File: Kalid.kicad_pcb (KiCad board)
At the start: 4 copper layers, 90 x 40 mm, 160 parts, among them J1 USB_A, J2 USB_C_Receptacle_USB2.0_16P, J3 USB_A, J31 DC Connector, J4 USB_A, J5 USB_A, J6 Conn_01x04, J7 USB_C_Receptacle_USB2.0_16P, U1 TPS62933, U2 TPS62933, U3 GL3523-OTY30, U4 USB-PD, U5 LPW5209AB5F, U6 LPW5209AB5F, U7 LPW5209AB5F, U8 LPW5209AB5F, U9 MX25L1006EMI-10G, Y1 Crystal 25MHz 2016

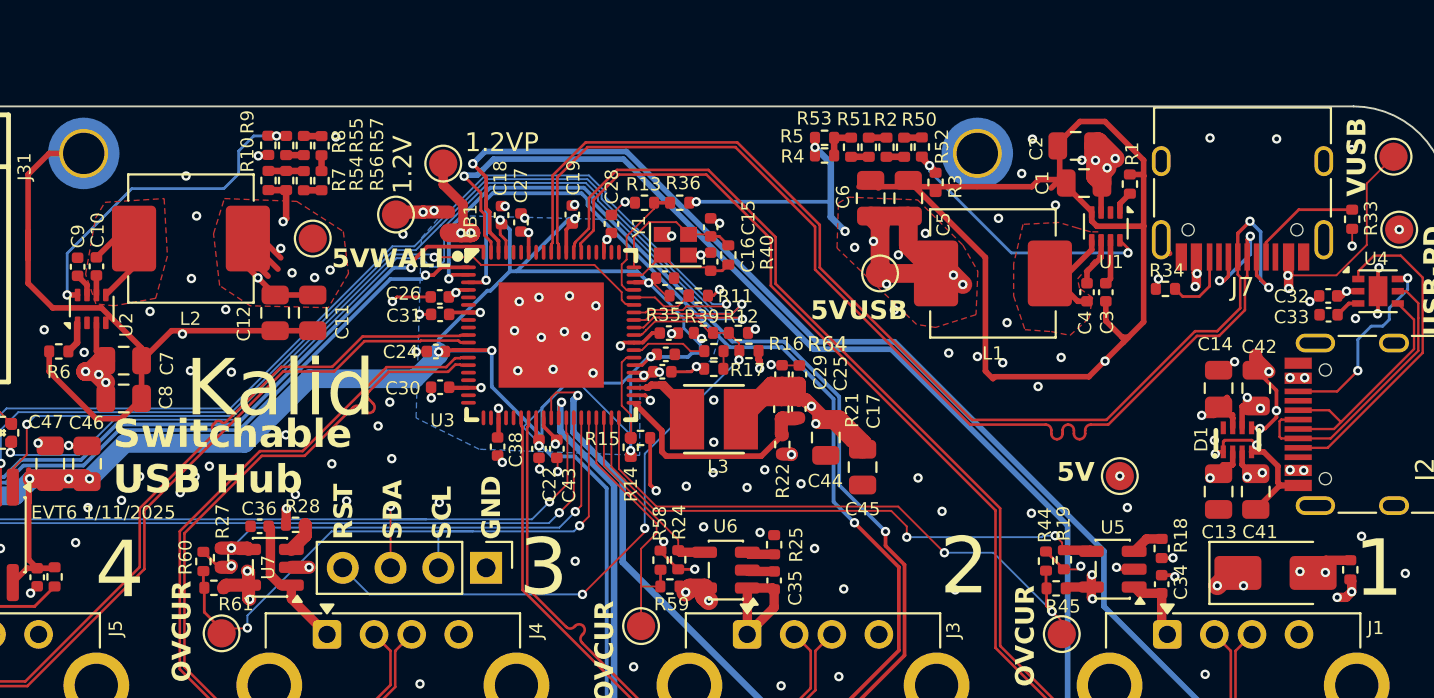
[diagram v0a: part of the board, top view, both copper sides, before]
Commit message: evt5: Release
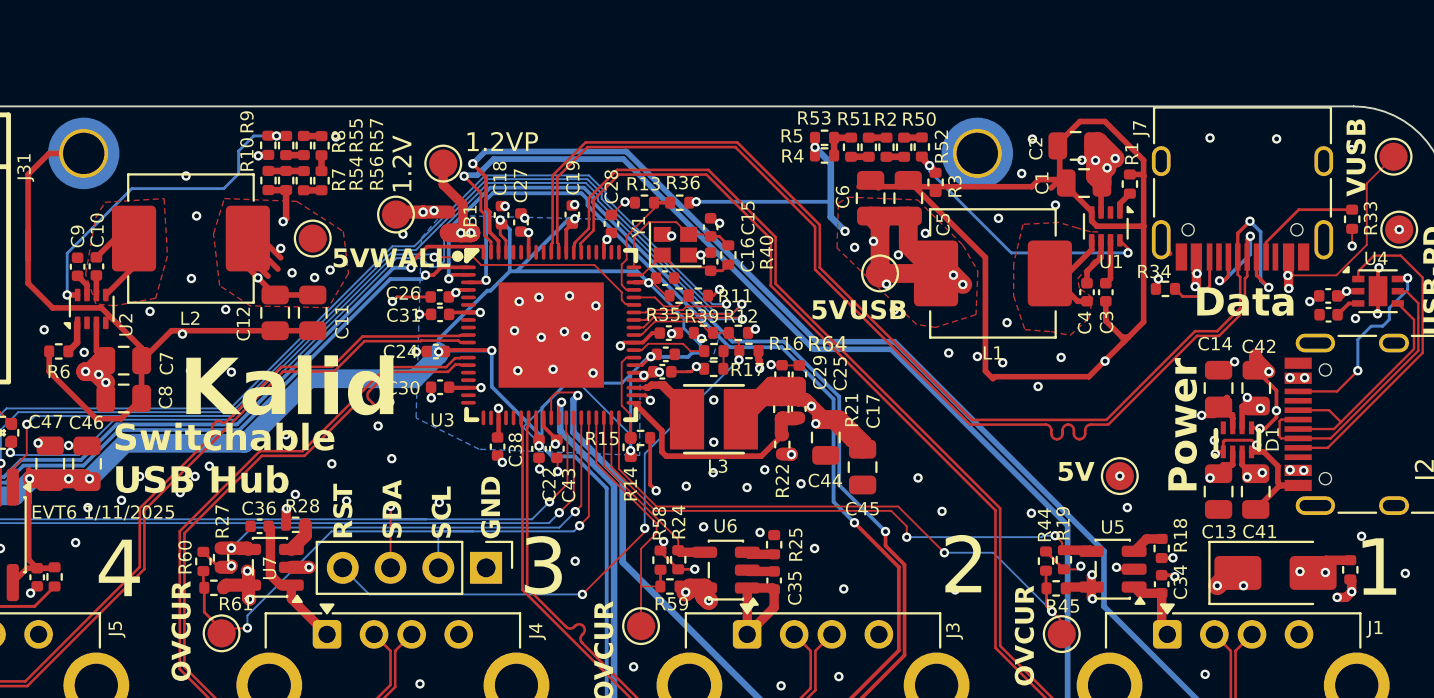
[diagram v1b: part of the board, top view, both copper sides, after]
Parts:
- R20, R23, R26, R29: value R 510 0402 -> R 1k 0402
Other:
- board text added: "Data"
- board text added: "Power"
